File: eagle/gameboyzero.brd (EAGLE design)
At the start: 71 x 89 mm, 22 parts

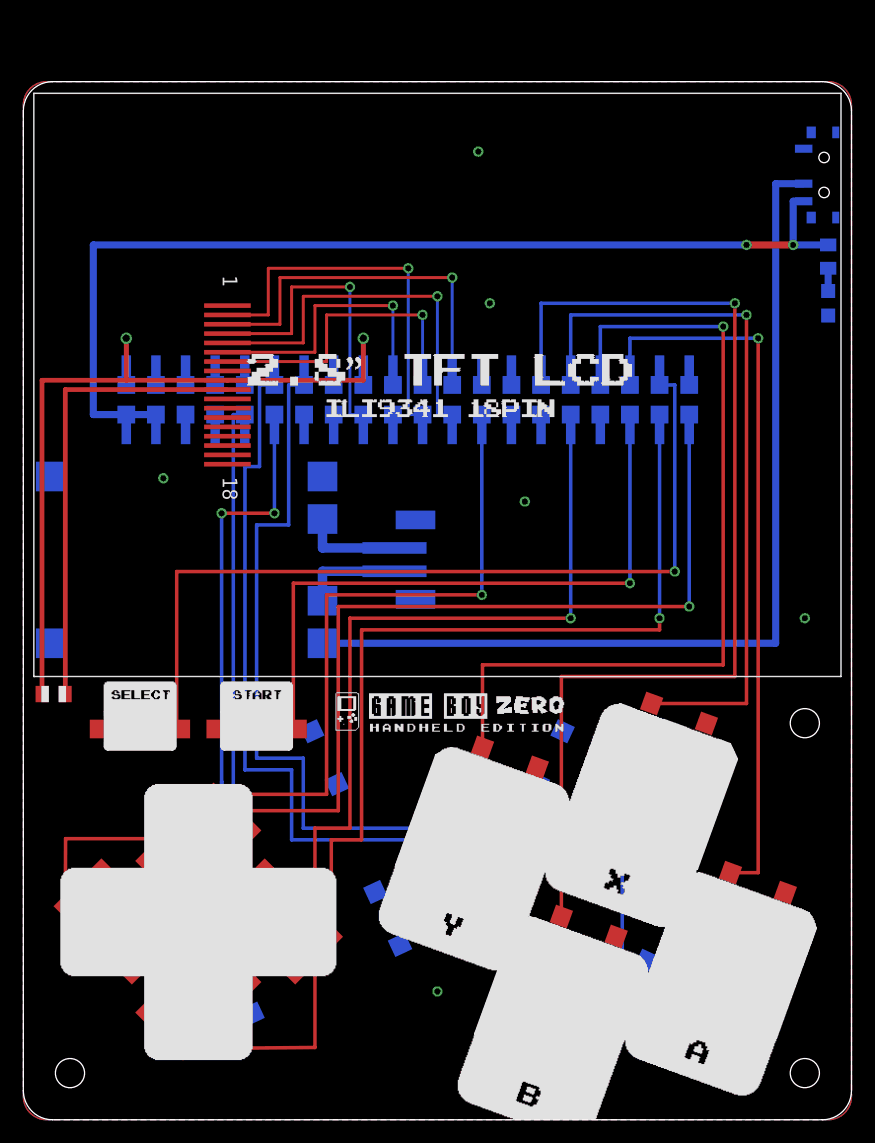
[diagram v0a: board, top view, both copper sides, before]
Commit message: New Silk and New Case files
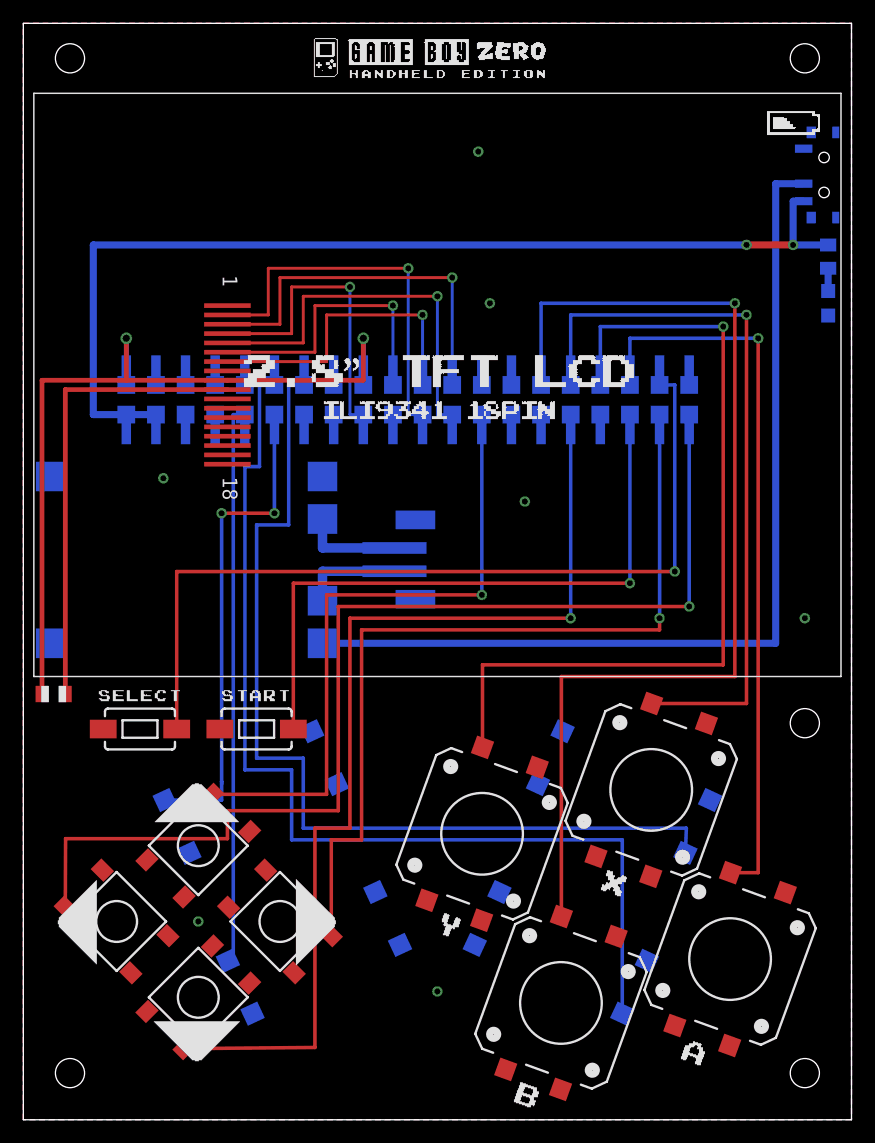
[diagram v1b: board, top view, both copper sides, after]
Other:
- board size 71 x 89 mm -> 71 x 94 mm

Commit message: Fri 13 Oct 2017 16:15:10 EDT
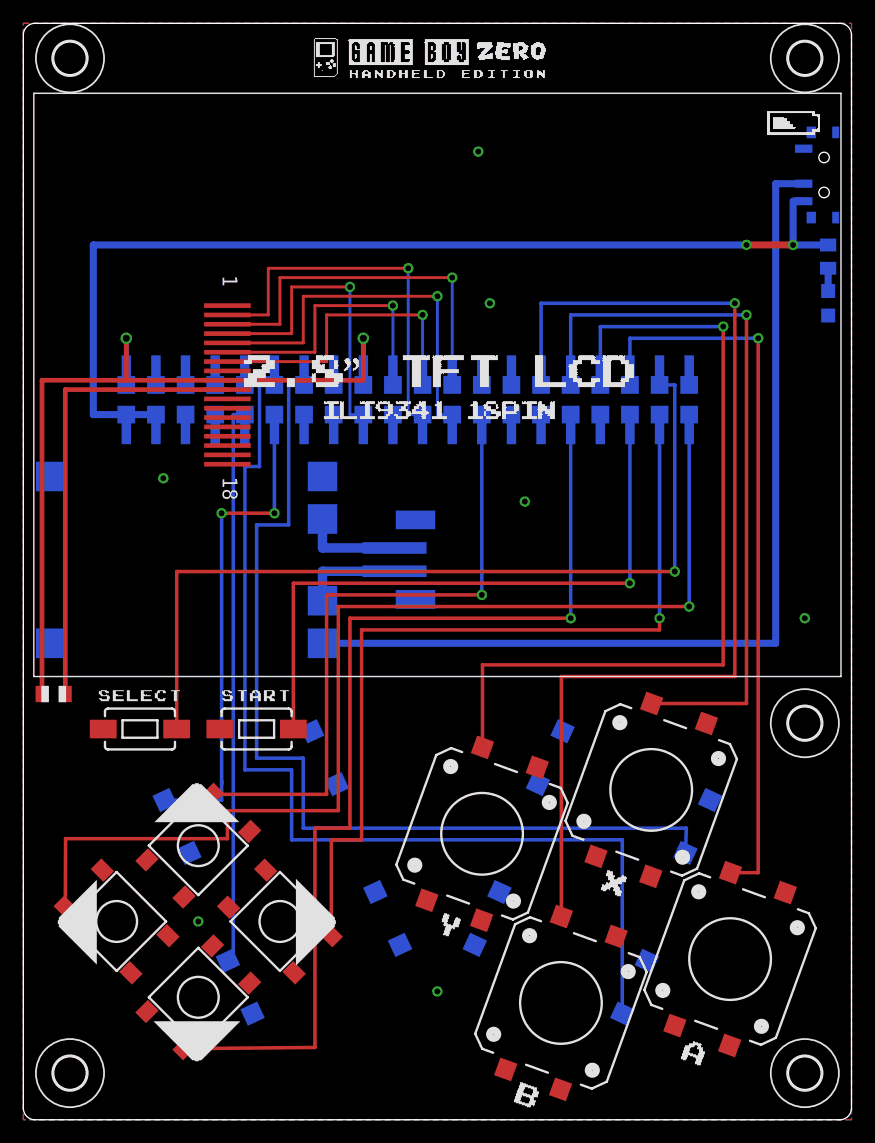
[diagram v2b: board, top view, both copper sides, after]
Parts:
- added H1, H2, H3, H4, H5: MOUNT-HOLE2.8, holes:2,8
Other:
- outline, holes or cut-outs redrawn
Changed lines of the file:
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@@
 <setting verticaltext="up"/>
 </settings>
-<grid distance="0.08575" unitdist="mm" unit="mm" style="lines" multiple="1" display="yes" altdistance="0.25" altunitdist="mm" altunit="mm"/>
+<grid distance="1" unitdist="mm" unit="mm" style="lines" multiple="1" display="yes" altdistance="0.25" altunitdist="mm" altunit="mm"/>
 <layers>
 <layer number="1" name="Top" color="4" fill="1" visible="yes" active="yes"/>
@@
 <board>
 <plain>
-<wire x1="71" y1="94" x2="0" y2="94" width="0" layer="20"/>
-<wire x1="0" y1="94" x2="0" y2="0" width="0" layer="20"/>
-<wire x1="0" y1="0" x2="71" y2="0" width="0" layer="20"/>
-<wire x1="71" y1="0" x2="71" y2="94" width="0" layer="20"/>
+<wire x1="0" y1="93" x2="0" y2="1" width="0" layer="20"/>
+<wire x1="0" y1="1" x2="1" y2="0" width="0" layer="20" curve="90"/>
+<wire x1="1" y1="0" x2="70" y2="0" width="0" layer="20"/>
+<wire x1="70" y1="0" x2="71" y2="1" width="0" layer="20" curve="90"/>
+<wire x1="71" y1="1" x2="71" y2="93" width="0" layer="20"/>
+<wire x1="71" y1="93" x2="70" y2="94" width="0" layer="20" curve="90"/>
+<wire x1="70" y1="94" x2="1" y2="94" width="0" layer="20"/>
+<wire x1="1" y1="94" x2="0" y2="93" width="0" layer="20" curve="90"/>
 <rectangle x1="0" y1="0" x2="62" y2="77" layer="222"/>
 <rectangle x1="0" y1="0" x2="62" y2="77" layer="222"/>
@@
 <rectangle x1="0" y1="0" x2="71" y2="89" layer="222"/>
 <rectangle x1="0" y1="0" x2="71" y2="89" layer="222"/>
-<circle x="67" y="34" radius="1.25" width="0.01" layer="20"/>
-<circle x="67" y="4" radius="1.25" width="0.01" layer="20"/>
-<circle x="4" y="4" radius="1.25" width="0.01" layer="20"/>
-<circle x="67" y="91" radius="1.25" width="0.01" layer="20"/>
-<circle x="4" y="91" radius="1.25" width="0.01" layer="20"/>
 <rectangle x1="43.1751" y1="1.07188125" x2="43.5181" y2="1.15763125" layer="21"/>
 <rectangle x1="43.0036" y1="1.15763125" x2="43.5181" y2="1.24338125" layer="21"/>
@@
 <attribute name="SF_SKU" value="COM-12992" x="22" y="17" size="1.778" layer="27" rot="R315" display="off"/>
 </element>
+<element name="H1" library="holes" library_urn="urn:adsk.eagle:library:237" package="2,8" package3d_urn="urn:adsk.eagle:package:14271/1" value="MOUNT-HOLE2.8" x="4" y="4"/>
+<element name="H2" library="holes" library_urn="urn:adsk.eagle:library:237" package="2,8" package3d_urn="urn:adsk.eagle:package:14271/1" value="MOUNT-HOLE2.8" x="67" y="4"/>
+<element name="H3" library="holes" library_urn="urn:adsk.eagle:library:237" package="2,8" package3d_urn="urn:adsk.eagle:package:14271/1" value="MOUNT-HOLE2.8" x="67" y="34"/>
+<element name="H4" library="holes" library_urn="urn:adsk.eagle:library:237" package="2,8" package3d_urn="urn:adsk.eagle:package:14271/1" value="MOUNT-HOLE2.8" x="4" y="91"/>
+<element name="H5" library="holes" library_urn="urn:adsk.eagle:library:237" package="2,8" package3d_urn="urn:adsk.eagle:package:14271/1" value="MOUNT-HOLE2.8" x="67" y="91"/>
 </elements>
 <signals>
